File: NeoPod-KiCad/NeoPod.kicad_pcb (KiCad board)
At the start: 4 copper layers, 100 x 120 mm, 62 parts, among them J1 SJ-3523-SMT-TR, J2 USB4500-03-0-A_REVA1, J4 USB4500-03-0-A_REVA1, Q1 CSD25480F3, SW1 SW_SPST, SW2 SW_SPST, SW3 SW_SPST, SW4 SW_SPST, SW5 SW_SPST, U1 ESP32-WROOM-32, U10 SN74CB3Q3257DBQR, U2 PCM5102A, U3 RP2040, U4 CP2102N-Axx-xQFN24, U5 XC6210B332MR, U6 STC4054GR, U7 TFT_320x240, Y2 40MHz-Xtal

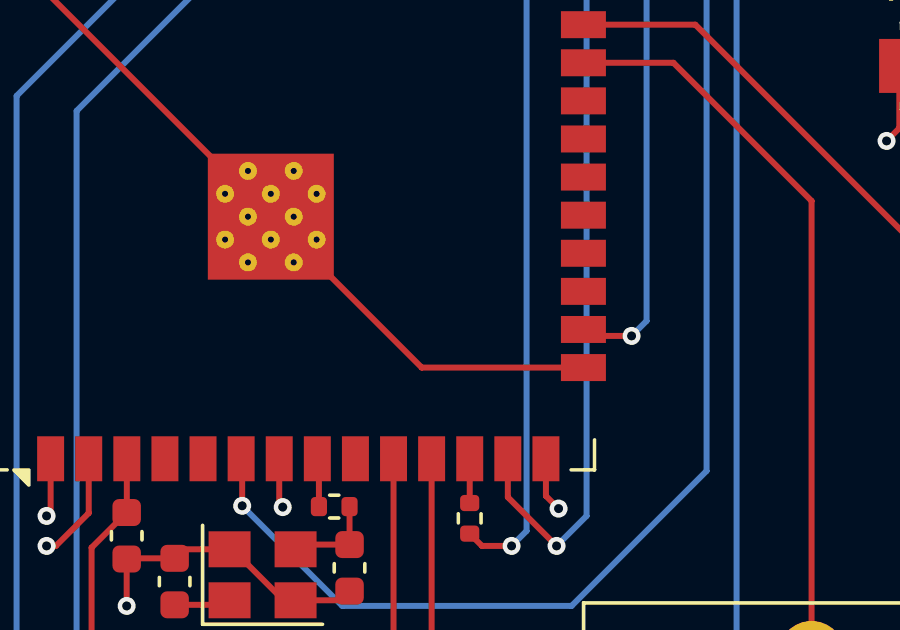
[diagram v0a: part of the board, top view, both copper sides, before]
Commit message: finished pcb
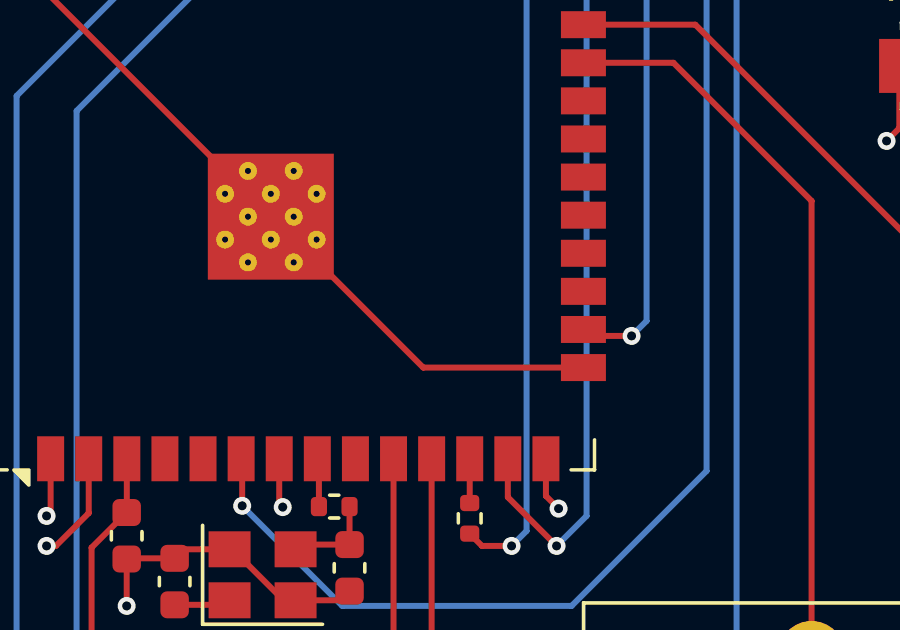
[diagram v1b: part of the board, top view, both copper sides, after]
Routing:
- net DIN: track 113.7 -> 115.5 mm
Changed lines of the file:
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@@
+	)
+	(segment
+		(start 129.895 96.555)
+		(end 124.555 96.555)
+		(width 0.2)
+		(layer "F.Cu")
+		(net 89)
 	)
 	(segment
@@
 	)
 	(segment
+		(start 121.05 93.05)
+		(end 121 93.05)
+		(width 0.2)
+		(layer "F.Cu")
+		(net 89)
+	)
+	(segment
 		(start 129.55 137.212858)
 		(end 129.55 135.461171)
@@
 	)
 	(segment
-		(start 124.505 96.555)
-		(end 121 93.05)
-		(width 0.2)
-		(layer "F.Cu")
-		(net 89)
-	)
-	(segment
 		(start 116.268915 102.913304)
 		(end 114.693467 102.913304)
@@
 	)
 	(segment
-		(start 129.895 96.555)
-		(end 124.505 96.555)
-		(width 0.2)
-		(layer "F.Cu")
-		(net 89)
-	)
-	(segment
 		(start 189.936718 118.563282)
 		(end 188.5 120)
@@
 	)
 	(segment
+		(start 124.555 96.555)
+		(end 121.05 93.05)
+		(width 0.2)
+		(layer "F.Cu")
+		(net 89)
+	)
+	(segment
 		(start 189.986718 118.180712)
 		(end 189.936718 118.230712)
@@
 	)
 	(segment
-		(start 114.5 98)
+		(start 114.5 101)
 		(end 114.5 80)
 		(width 0.2)
@@
 	)
 	(segment
-		(start 125 108.5)
-		(end 114.5 98)
+		(start 155.9 142.4)
+		(end 114.5 101)
 		(width 0.2)
 		(layer "In1.Cu")
@@
 	)
 	(segment
-		(start 158.9 142.4)
-		(end 125 108.5)
+		(start 188 142.4)
+		(end 155.9 142.4)
 		(width 0.2)
 		(layer "In1.Cu")
-		(net 114)
-	)
-	(segment
-		(start 188 142.4)
-		(end 158.9 142.4)
-		(width 0.2)
-		(layer "In1.Cu")
